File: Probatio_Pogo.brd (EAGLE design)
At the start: 21.5 x 8 mm, 5 parts

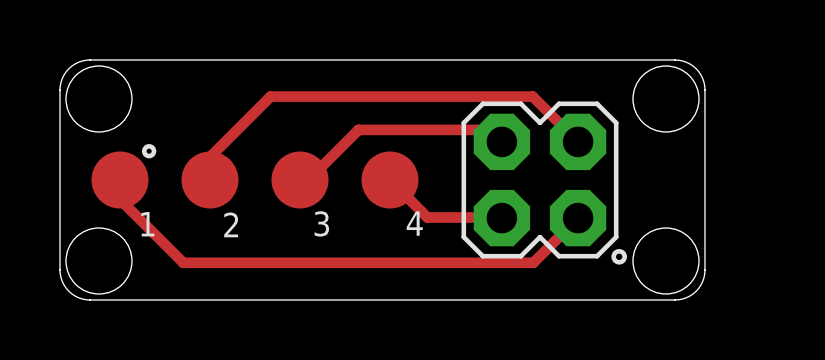
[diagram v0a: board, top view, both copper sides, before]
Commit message: Update Probatio_Pogo.brd
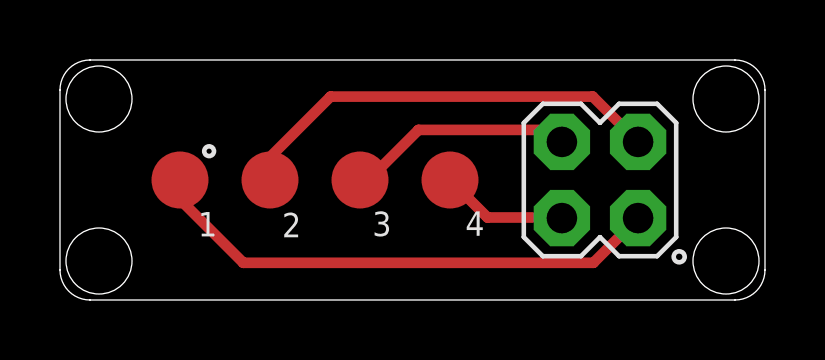
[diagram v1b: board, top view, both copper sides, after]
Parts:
- moved POGO1 2.00 mm to (4.00, 4.00)
- moved POGO2 2.00 mm to (7.00, 4.00)
- moved POGO3 2.00 mm to (10.0, 4.00)
- moved POGO4 2.00 mm to (13.0, 4.00)
- moved U$1 2.00 mm to (18.0, 4.00)
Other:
- board size 21.5 x 8 mm -> 23.5 x 8 mm
- board text added: "pogo-pcb v0.2.0"
- board text added: "probatio"
- board text removed: "Pogo-board v0.2.0"
- board text removed: "Probatio"
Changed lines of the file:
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@@
 <board>
 <plain>
-<wire x1="21.5" y1="1" x2="21.5" y2="7" width="0" layer="20"/>
+<wire x1="23.5" y1="1" x2="23.5" y2="7" width="0" layer="20"/>
 <wire x1="0" y1="7" x2="0" y2="1" width="0" layer="20"/>
-<wire x1="20.5" y1="8" x2="1" y2="8" width="0" layer="20"/>
-<text x="2.6" y="2.12" size="0.8128" layer="21" font="vector">1</text>
-<text x="5.4" y="2.09" size="0.8128" layer="21" font="vector">2</text>
-<text x="8.41" y="2.13" size="0.8128" layer="21" font="vector">3</text>
-<text x="11.51" y="2.14" size="0.8128" layer="21" font="vector">4</text>
-<text x="19.33" y="2.32" size="0.8128" layer="22" font="vector" rot="MR0">1</text>
-<text x="19.35" y="4.88" size="0.8128" layer="22" font="vector" rot="MR0">2</text>
-<text x="13.1" y="4.9" size="0.8128" layer="22" font="vector" rot="MR0">3</text>
-<text x="13.1" y="2.44" size="0.8128" layer="22" font="vector" rot="MR0">4</text>
-<wire x1="1" y1="0" x2="20.5" y2="0" width="0" layer="20"/>
+<wire x1="22.5" y1="8" x2="1" y2="8" width="0" layer="20"/>
+<text x="4.6" y="2.12" size="0.8128" layer="21" font="vector">1</text>
+<text x="7.4" y="2.09" size="0.8128" layer="21" font="vector">2</text>
+<text x="10.41" y="2.13" size="0.8128" layer="21" font="vector">3</text>
+<text x="13.51" y="2.14" size="0.8128" layer="21" font="vector">4</text>
+<text x="21.33" y="2.32" size="0.8128" layer="22" font="vector" rot="MR0">1</text>
+<text x="21.35" y="4.88" size="0.8128" layer="22" font="vector" rot="MR0">2</text>
+<text x="15.1" y="4.9" size="0.8128" layer="22" font="vector" rot="MR0">3</text>
+<text x="15.1" y="2.44" size="0.8128" layer="22" font="vector" rot="MR0">4</text>
+<wire x1="1" y1="0" x2="22.5" y2="0" width="0" layer="20"/>
 <wire x1="0" y1="7" x2="1" y2="8" width="0" layer="20" curve="-90"/>
 <wire x1="0" y1="1" x2="1" y2="0" width="0" layer="20" curve="90"/>
-<wire x1="20.5" y1="0" x2="21.5" y2="1" width="0" layer="20" curve="90"/>
-<wire x1="21.5" y1="7" x2="20.5" y2="8" width="0" layer="20" curve="90"/>
-<hole x="20.2" y="1.3" drill="2.2"/>
-<hole x="20.2" y="6.7" drill="2.2"/>
+<wire x1="22.5" y1="0" x2="23.5" y2="1" width="0" layer="20" curve="90"/>
+<wire x1="23.5" y1="7" x2="22.5" y2="8" width="0" layer="20" curve="90"/>
+<hole x="22.2" y="1.3" drill="2.2"/>
+<hole x="22.2" y="6.7" drill="2.2"/>
 <hole x="1.3" y="6.7" drill="2.2"/>
 <hole x="1.3" y="1.3" drill="2.2"/>
-<circle x="18.64" y="1.44" radius="0.183575" width="0.1524" layer="21"/>
-<circle x="2.97" y="4.96" radius="0.1627875" width="0.1524" layer="21"/>
-<text x="11.84" y="3.3" size="1.778" layer="22" font="vector" rot="MR0">Probatio</text>
-<text x="12" y="1" size="0.6096" layer="22" font="vector" rot="MR0">Pogo-board v0.2.0</text>
+<circle x="20.64" y="1.44" radius="0.183575" width="0.1524" layer="21"/>
+<circle x="4.97" y="4.96" radius="0.1627875" width="0.1524" layer="21"/>
+<text x="13.84" y="3.3" size="1.778" layer="22" font="vector" rot="MR0">probatio</text>
+<text x="14" y="1" size="0.6096" layer="22" font="vector" rot="MR0">pogo-pcb v0.2.0</text>
 </plain>
 <attributes>
@@
 </autorouter>
 <elements>
-<element name="POGO1" library="Batebit" package="POGO_PIN" value="POGO_PIN0900-0-15-20-76-14-11-0" x="2" y="4"/>
-<element name="POGO2" library="Batebit" package="POGO_PIN" value="POGO_PIN0900-0-15-20-76-14-11-0" x="5" y="4"/>
-<element name="POGO3" library="Batebit" package="POGO_PIN" value="POGO_PIN0900-0-15-20-76-14-11-0" x="8" y="4"/>
-<element name="POGO4" library="Batebit" package="POGO_PIN" value="POGO_PIN0900-0-15-20-76-14-11-0" x="11" y="4"/>
-<element name="U$1" library="Batebit" package="2X2" value="M02X22X2" x="16" y="4"/>
+<element name="POGO1" library="Batebit" package="POGO_PIN" value="POGO_PIN0900-0-15-20-76-14-11-0" x="4" y="4"/>
+<element name="POGO2" library="Batebit" package="POGO_PIN" value="POGO_PIN0900-0-15-20-76-14-11-0" x="7" y="4"/>
+<element name="POGO3" library="Batebit" package="POGO_PIN" value="POGO_PIN0900-0-15-20-76-14-11-0" x="10" y="4"/>
+<element name="POGO4" library="Batebit" package="POGO_PIN" value="POGO_PIN0900-0-15-20-76-14-11-0" x="13" y="4"/>
+<element name="U$1" library="Batebit" package="2X2" value="M02X22X2" x="18" y="4"/>
 </elements>
 <signals>
@@
 <contactref element="POGO4" pad="P$1"/>
 <contactref element="U$1" pad="1"/>
-<wire x1="11" y1="4" x2="12.25" y2="2.75" width="0.3556" layer="1"/>
-<wire x1="12.25" y1="2.75" x2="14.71" y2="2.75" width="0.3556" layer="1"/>
-<wire x1="14.71" y1="2.75" x2="14.73" y2="2.73" width="0.3048" layer="1"/>
+<wire x1="13" y1="4" x2="14.25" y2="2.75" width="0.3556" layer="1"/>
+<wire x1="14.25" y1="2.75" x2="16.71" y2="2.75" width="0.3556" layer="1"/>
+<wire x1="16.71" y1="2.75" x2="16.73" y2="2.73" width="0.3048" layer="1"/>
 </signal>
 <signal name="P1">
 <contactref element="POGO1" pad="P$1"/>
 <contactref element="U$1" pad="3"/>
-<wire x1="2" y1="4" x2="2" y2="3.35" width="0.3556" layer="1"/>
-<wire x1="2" y1="3.35" x2="4.11" y2="1.24" width="0.3556" layer="1"/>
-<wire x1="4.11" y1="1.24" x2="15.78" y2="1.24" width="0.3556" layer="1"/>
-<wire x1="15.78" y1="1.24" x2="17.27" y2="2.73" width="0.3556" layer="1"/>
+<wire x1="4" y1="4" x2="4" y2="3.35" width="0.3556" layer="1"/>
+<wire x1="4" y1="3.35" x2="6.11" y2="1.24" width="0.3556" layer="1"/>
+<wire x1="6.11" y1="1.24" x2="17.78" y2="1.24" width="0.3556" layer="1"/>
+<wire x1="17.78" y1="1.24" x2="19.27" y2="2.73" width="0.3556" layer="1"/>
 </signal>
 <signal name="P2">
 <contactref element="POGO2" pad="P$1"/>
 <contactref element="U$1" pad="4"/>
-<wire x1="5" y1="4" x2="5" y2="4.76" width="0.3556" layer="1"/>
-<wire x1="5" y1="4.76" x2="7.02" y2="6.78" width="0.3556" layer="1"/>
-<wire x1="7.02" y1="6.78" x2="15.76" y2="6.78" width="0.3556" layer="1"/>
-<wire x1="15.76" y1="6.78" x2="17.27" y2="5.27" width="0.3556" layer="1"/>
+<wire x1="7" y1="4" x2="7" y2="4.76" width="0.3556" layer="1"/>
+<wire x1="7" y1="4.76" x2="9.02" y2="6.78" width="0.3556" layer="1"/>
+<wire x1="9.02" y1="6.78" x2="17.76" y2="6.78" width="0.3556" layer="1"/>
+<wire x1="17.76" y1="6.78" x2="19.27" y2="5.27" width="0.3556" layer="1"/>
 </signal>
 <signal name="P3">
 <contactref element="POGO3" pad="P$1"/>
 <contactref element="U$1" pad="2"/>
-<wire x1="8" y1="4" x2="8.28" y2="4" width="0.3556" layer="1"/>
-<wire x1="8.28" y1="4" x2="9.95" y2="5.67" width="0.3556" layer="1"/>
-<wire x1="9.95" y1="5.67" x2="14.33" y2="5.67" width="0.3556" layer="1"/>
-<wire x1="14.33" y1="5.67" x2="14.73" y2="5.27" width="0.3556" layer="1"/>
+<wire x1="10" y1="4" x2="10.28" y2="4" width="0.3556" layer="1"/>
+<wire x1="10.28" y1="4" x2="11.95" y2="5.67" width="0.3556" layer="1"/>
+<wire x1="11.95" y1="5.67" x2="16.33" y2="5.67" width="0.3556" layer="1"/>
+<wire x1="16.33" y1="5.67" x2="16.73" y2="5.27" width="0.3556" layer="1"/>
 </signal>
 </signals>
